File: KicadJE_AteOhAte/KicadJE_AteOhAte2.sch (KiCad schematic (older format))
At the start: 63 parts, among them J201 In_Accent, J202 In Gate, J203 Out Final, P201 Doepfer_Power_10pin, Q201 MMBT2222A, Q202 MMBT2222A, Q203 MMBT2222A, Q204 MMBT2222A, SW201 Out 1, U201 TL072, U202 TL072

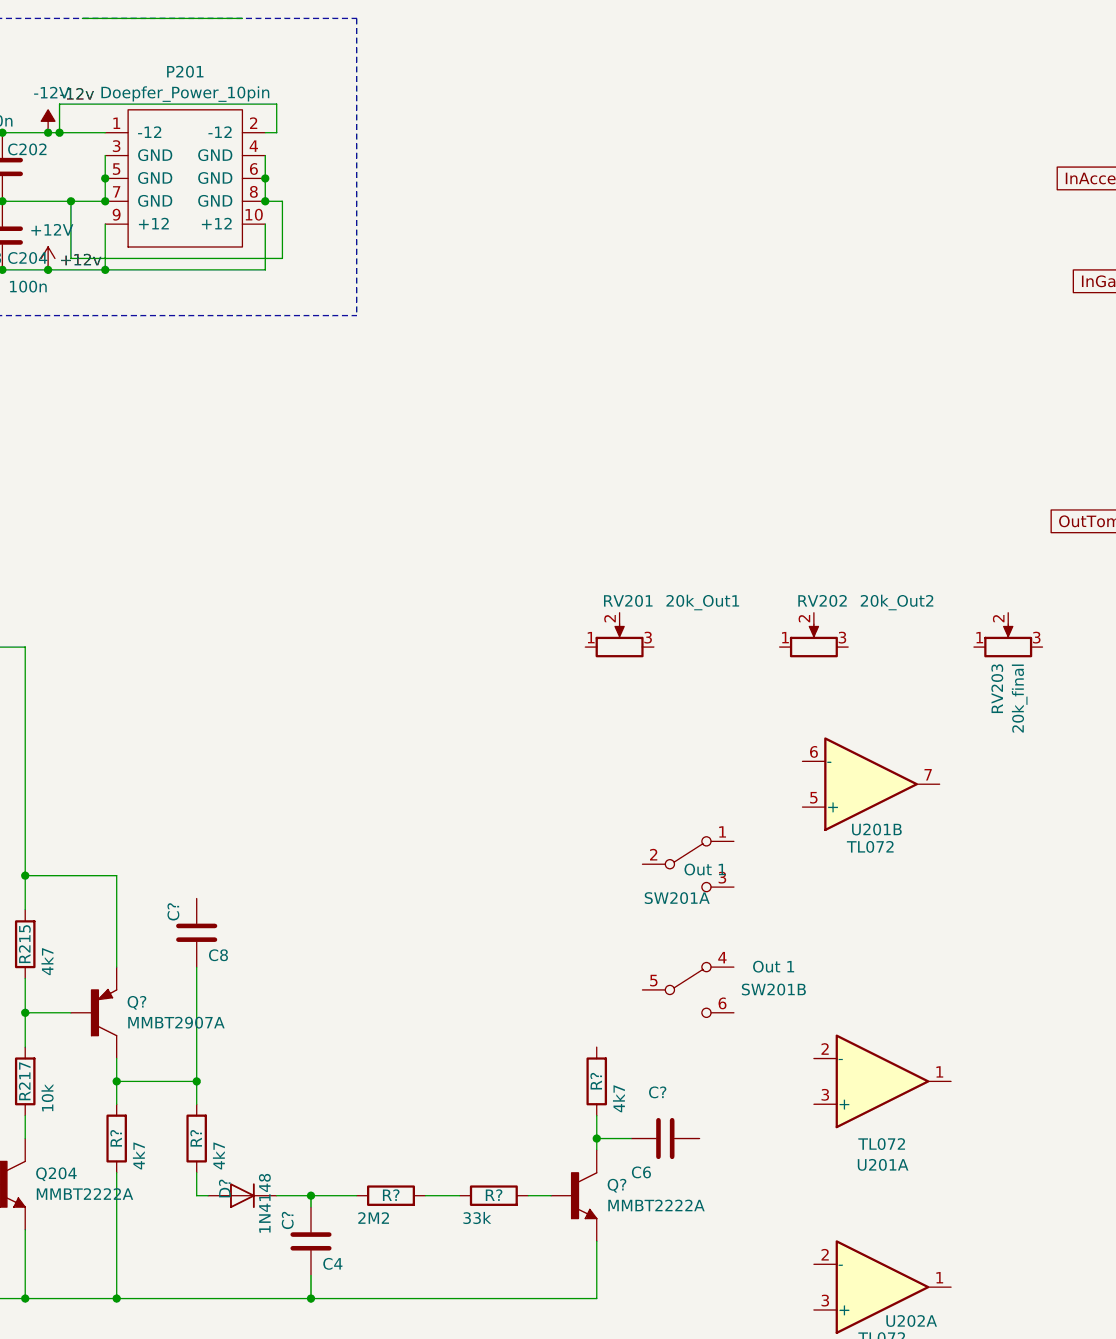
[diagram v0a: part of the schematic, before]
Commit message: 2nd
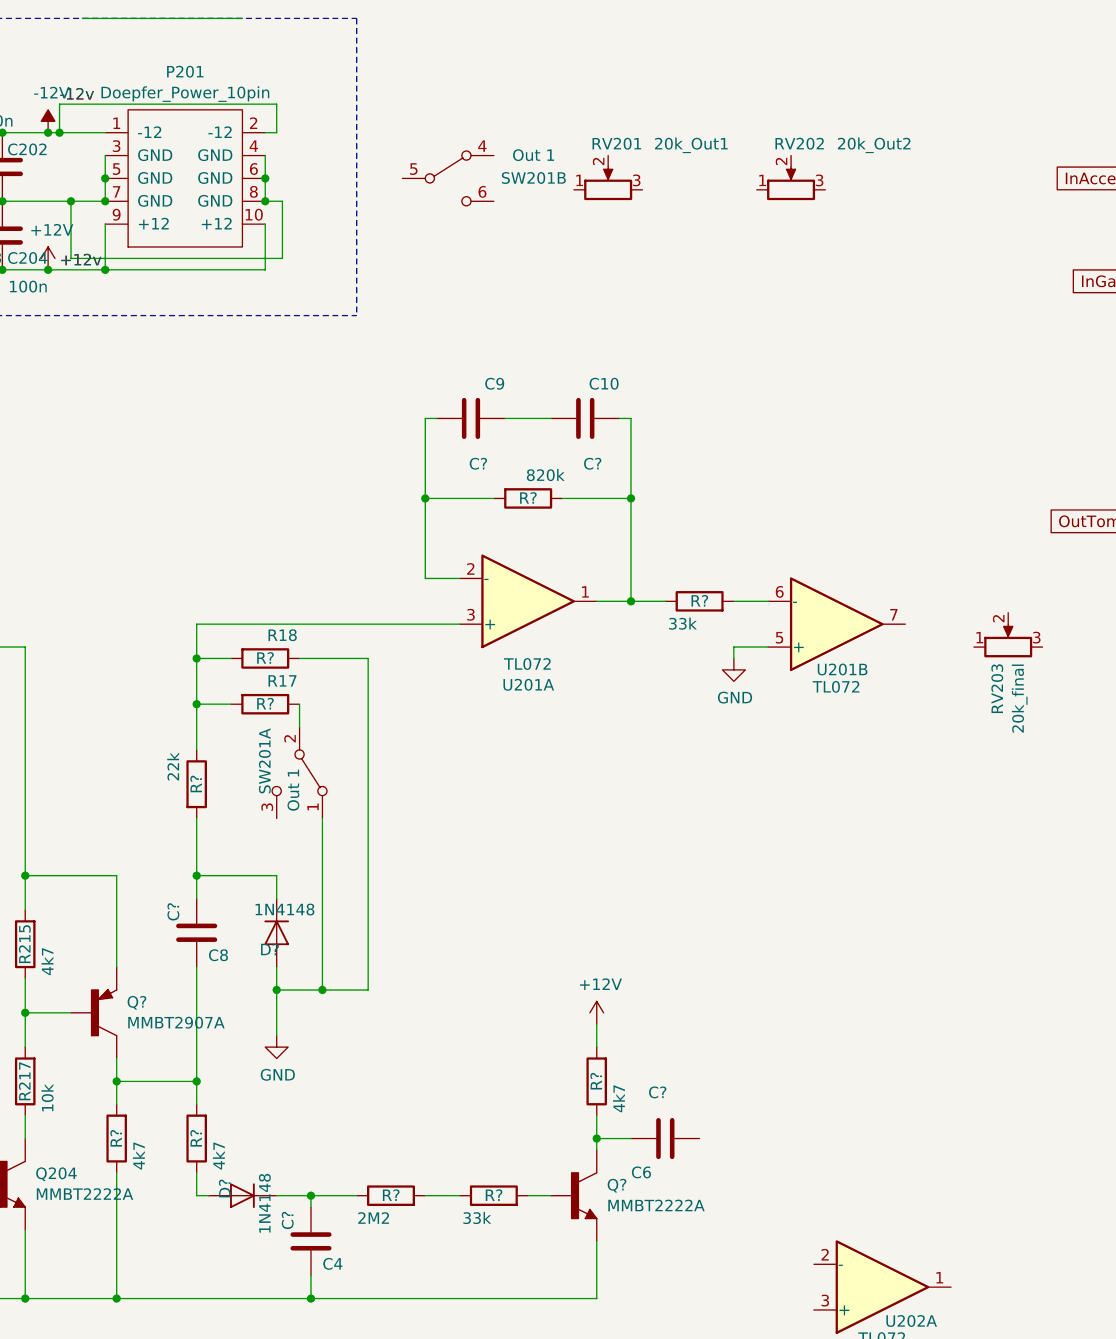
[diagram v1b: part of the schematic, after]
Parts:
- added C?: C9, Capacitor_SMD:C_0805_2012Metric_Pad1.15x1.40mm_HandSolder, symbol Device:C
- added C?: C10, Capacitor_SMD:C_0805_2012Metric_Pad1.15x1.40mm_HandSolder, symbol Device:C
- added D?: 1N4148, Diode_SMD:D_SOD-123, symbol Device:D
- added R?: 22k, Resistor_SMD:R_0805_2012Metric_Pad1.15x1.40mm_HandSolder, symbol Device:R
- added R?: R17, Resistor_SMD:R_0805_2012Metric_Pad1.15x1.40mm_HandSolder, symbol Device:R
- added R?: R18, Resistor_SMD:R_0805_2012Metric_Pad1.15x1.40mm_HandSolder, symbol Device:R
- added R?: 820k, Resistor_SMD:R_0805_2012Metric_Pad1.15x1.40mm_HandSolder, symbol Device:R
- added R?: 33k, Resistor_SMD:R_0805_2012Metric_Pad1.15x1.40mm_HandSolder, symbol Device:R
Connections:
- net +12V: now also R?.2
- net GND: now also SW201.1 (A), U201.5 (+), D?.2 (A), R?.1
- net at U201.6 (-): now also R?.2
- net at U201.1: now also C?.2, R?.1, R?.1
- net at U201.2 (-): now also C?.1, R?.2
- net at U201.3 (+): now also R?.1, R?.2, R?.2
- net at SW201.2 (B): now also R?.1
- net at C?.1: now also D?.1 (K), R?.2
- new net: C?.1, C?.2
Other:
- moved on the sheet: RV201, RV202, SW201A, SW201B, U201A, U201B

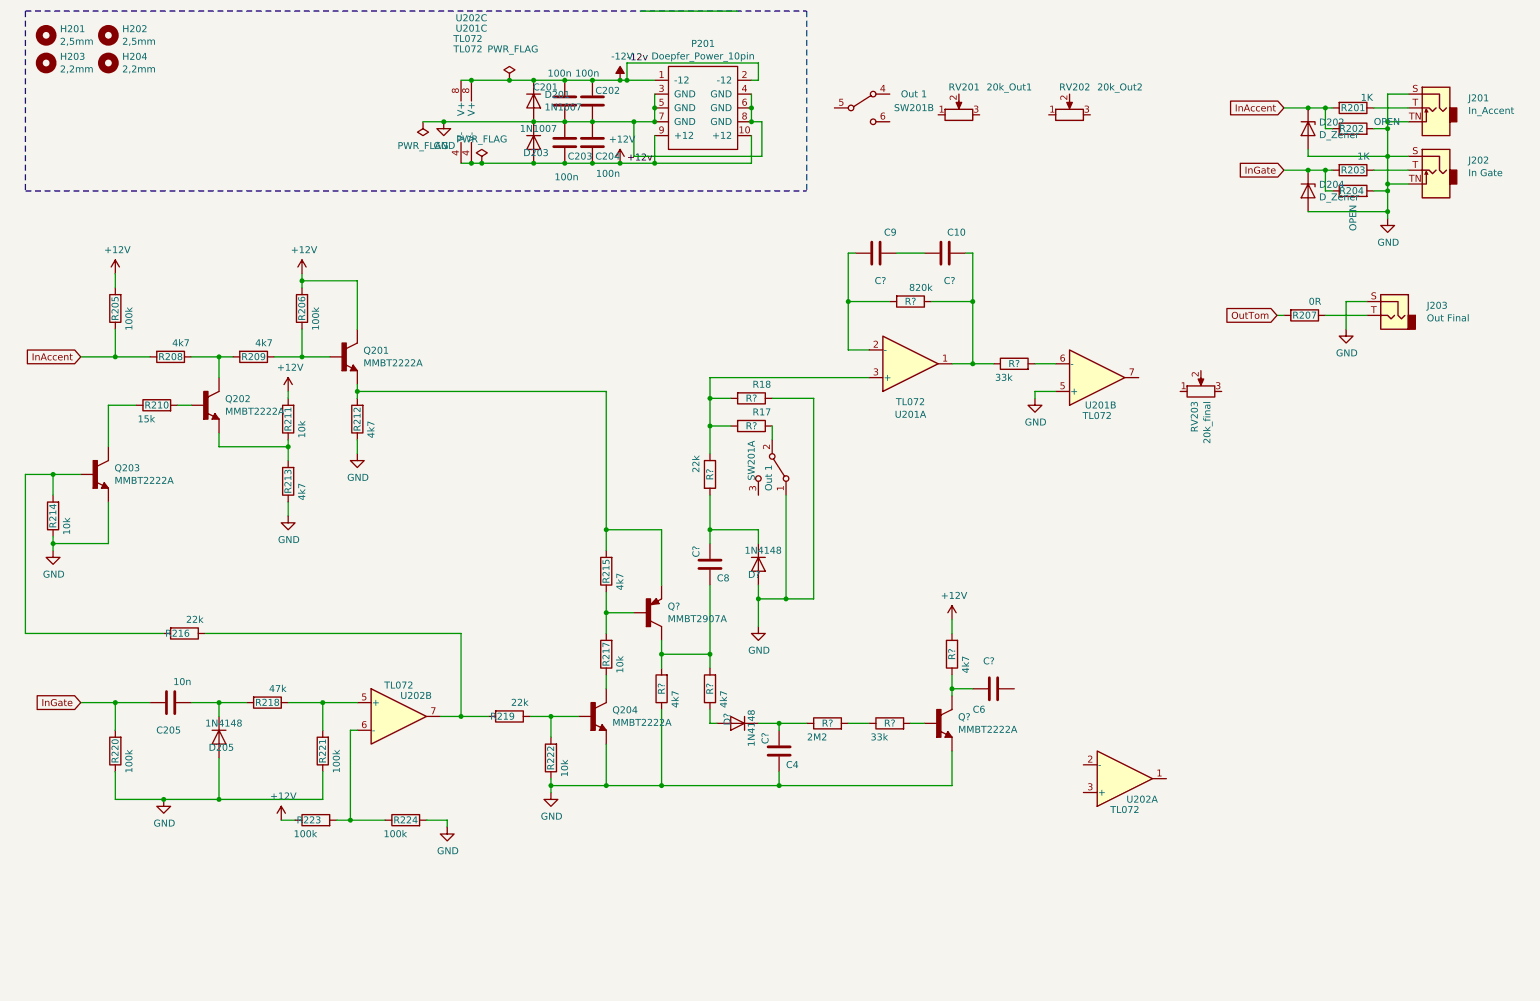
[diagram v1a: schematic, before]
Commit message: Initial SCH for the Tom
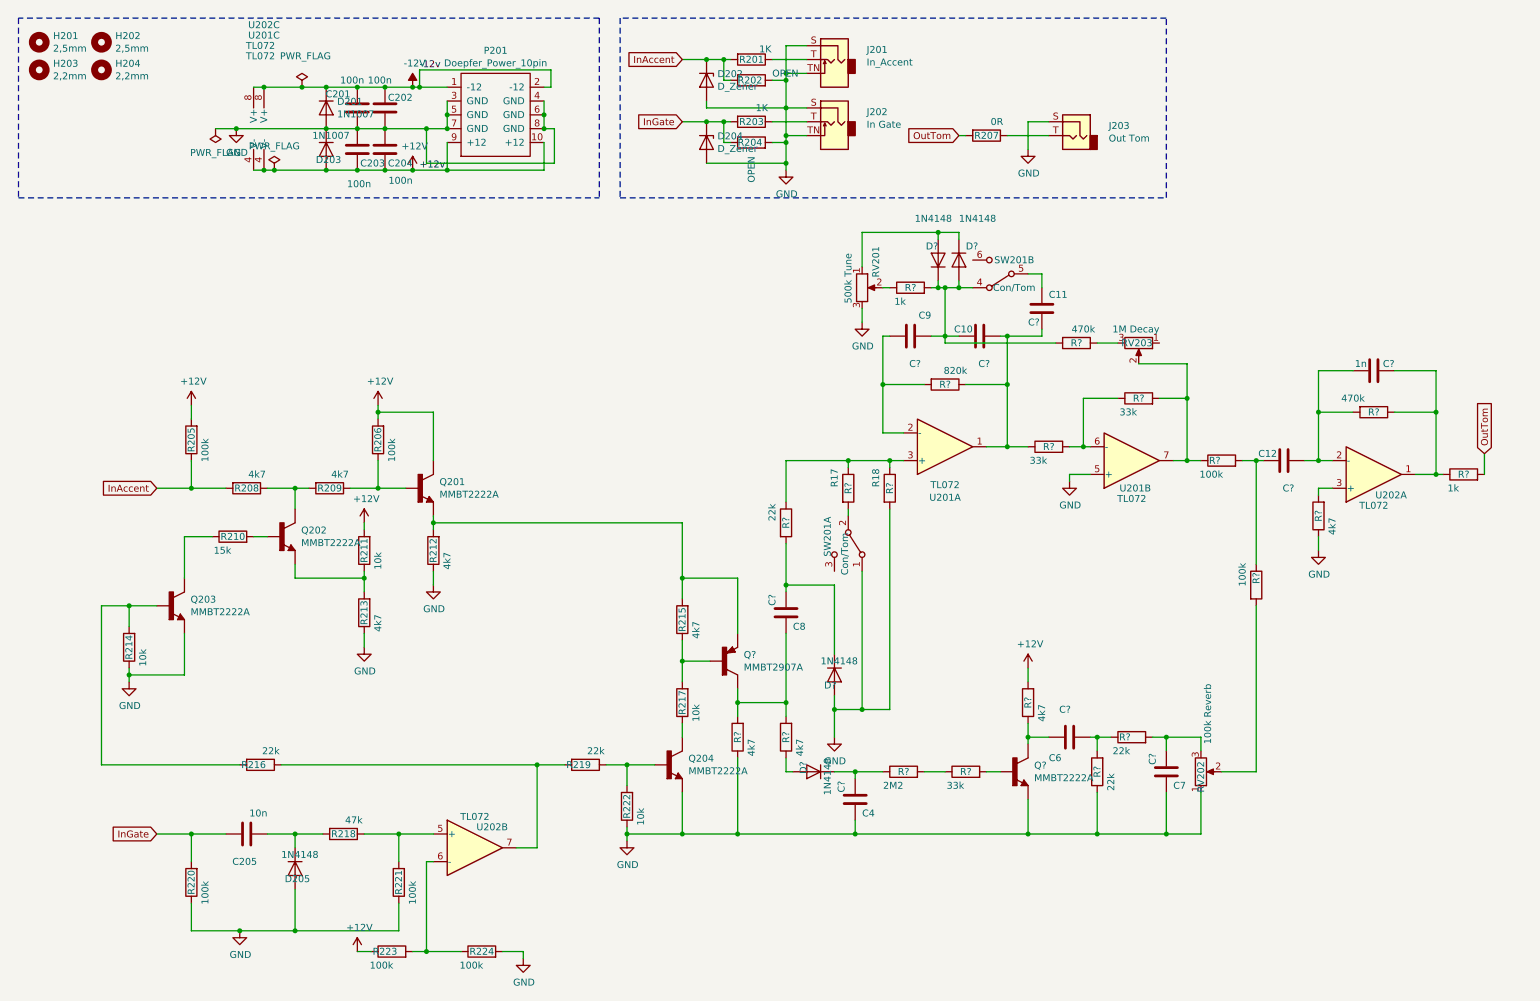
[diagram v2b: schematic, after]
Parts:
- added C?: C11, Capacitor_SMD:C_0805_2012Metric_Pad1.15x1.40mm_HandSolder, symbol Device:C
- added C?: C12, Capacitor_SMD:C_0805_2012Metric_Pad1.15x1.40mm_HandSolder, symbol Device:C
- added C?: 1n, Capacitor_SMD:C_0805_2012Metric_Pad1.15x1.40mm_HandSolder, symbol Device:C
- added C?: C7, Capacitor_SMD:C_0805_2012Metric_Pad1.15x1.40mm_HandSolder, symbol Device:C
- added D? (x2): 1N4148, Diode_SMD:D_SOD-123, symbol Device:D
- added R?: 33k, Resistor_SMD:R_0805_2012Metric_Pad1.15x1.40mm_HandSolder, symbol Device:R
- added R? (x2): 470k, Resistor_SMD:R_0805_2012Metric_Pad1.15x1.40mm_HandSolder, symbol Device:R
- added R? (x2): 1k, Resistor_SMD:R_0805_2012Metric_Pad1.15x1.40mm_HandSolder, symbol Device:R
- added R? (x2): 100k, Resistor_SMD:R_0805_2012Metric_Pad1.15x1.40mm_HandSolder, symbol Device:R
- added R?: 4k7, Resistor_SMD:R_0805_2012Metric_Pad1.15x1.40mm_HandSolder, symbol Device:R
- added R? (x2): 22k, Resistor_SMD:R_0805_2012Metric_Pad1.15x1.40mm_HandSolder, symbol Device:R
- J203: value Out Final -> Out Tom
- RV201: value 20k_Out1 -> 500k Tune
- RV202: value 20k_Out2 -> 100k Reverb
- RV203: value 20k_final -> 1M Decay
- SW201: value Out 1 -> Con/Tom
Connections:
- net GND: now also R?.2, RV201.3, RV202.1, C?.2, R?.1, R?.1; no longer R?.1
- net OutTom: now also R?.2
- net at U202.1: now also C?.2, R?.1, R?.1
- net at U202.2 (-): now also C?.1, C?.2, R?.2
- net at U202.3 (+): now also R?.2
- net at R?.2, U201.6 (-): now also R?.1
- net at U201.7: now also RV203.2, R?.1, R?.2
- net at RV203.3: now also R?.1
- net at RV201.1: now also D?.1 (K), D?.2 (A)
- net at RV201.2: now also R?.1
- net at C?.2, R?.1, R?.1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: now also C?.2
- net at R?.1, U201.3 (+): now also R?.1, R?.1; no longer R?.2, R?.2
- net at SW201.2 (B): now also R?.2; no longer R?.1
- net at SW201.4 (A): now also C?.1, C?.2, D?.1 (K), D?.2 (A), R?.2, R?.2
- net at SW201.5 (B): now also C?.1
- net at RV202.2: now also R?.2
- net at RV202.3: now also C?.1, R?.2
- net at C?.1: now also R?.1, R?.2
- new net: C?.1, R?.1, R?.2
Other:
- moved on the sheet: C201, C202, C203, C204, C205, C?, D201, D202, D203, D204, D205, D?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
